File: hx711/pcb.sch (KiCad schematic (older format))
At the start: 31 parts, among them J1 RJ45_LED, J2 CONN_02X03_Odd_Even, J3 CONN_02X03_Odd_Even, J4 CONN_02X03_Odd_Even, J5 CONN_02X03_Odd_Even, U1 sp485, U2 RS485, U3 RS485, U4 20M, U5 MIC55, U6 USBLC6-4SC6, U7 USBLC6-4SC6

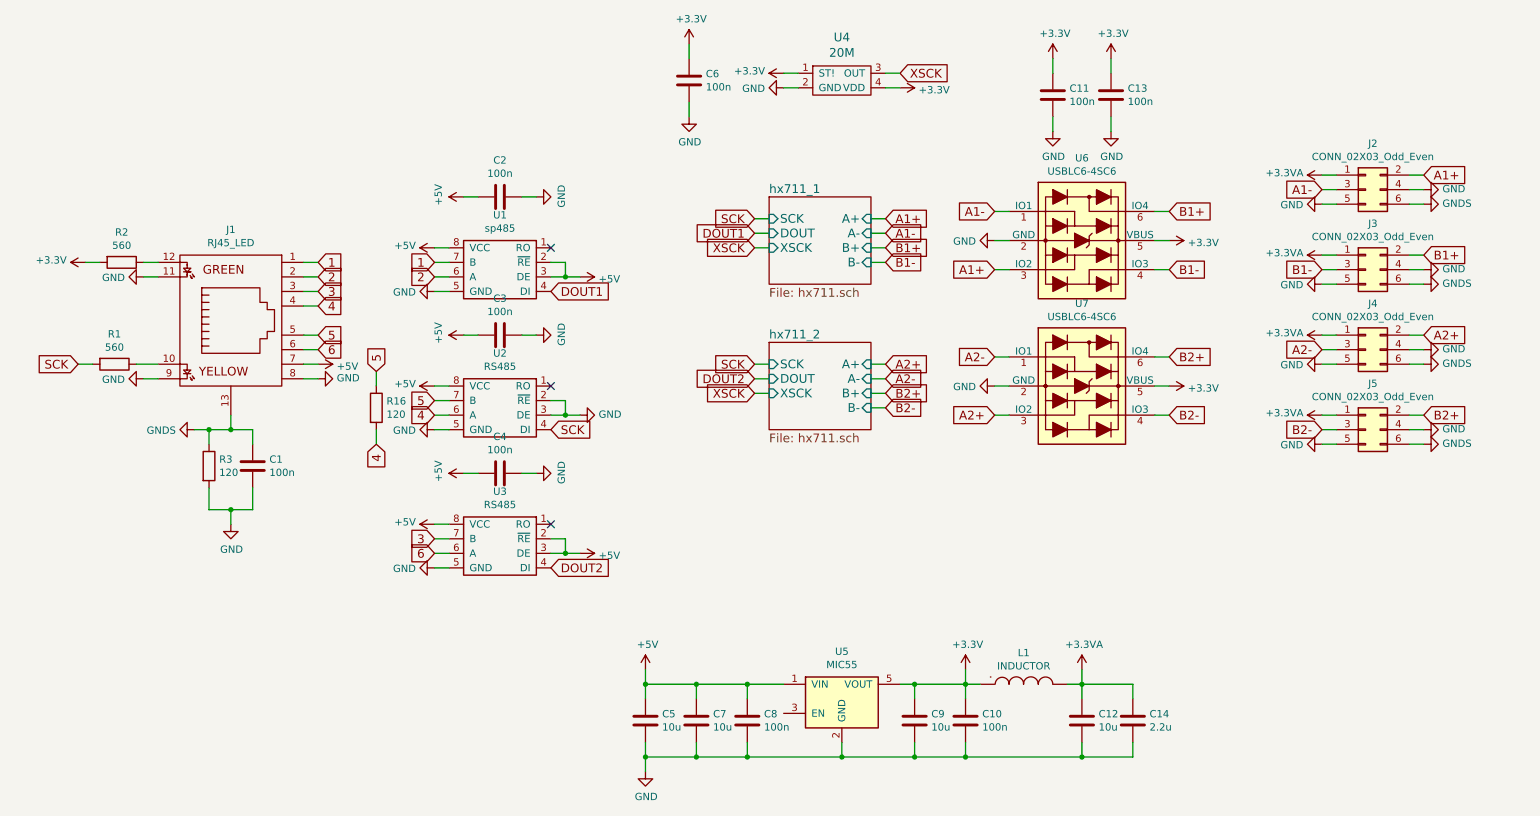
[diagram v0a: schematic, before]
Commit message: hx711
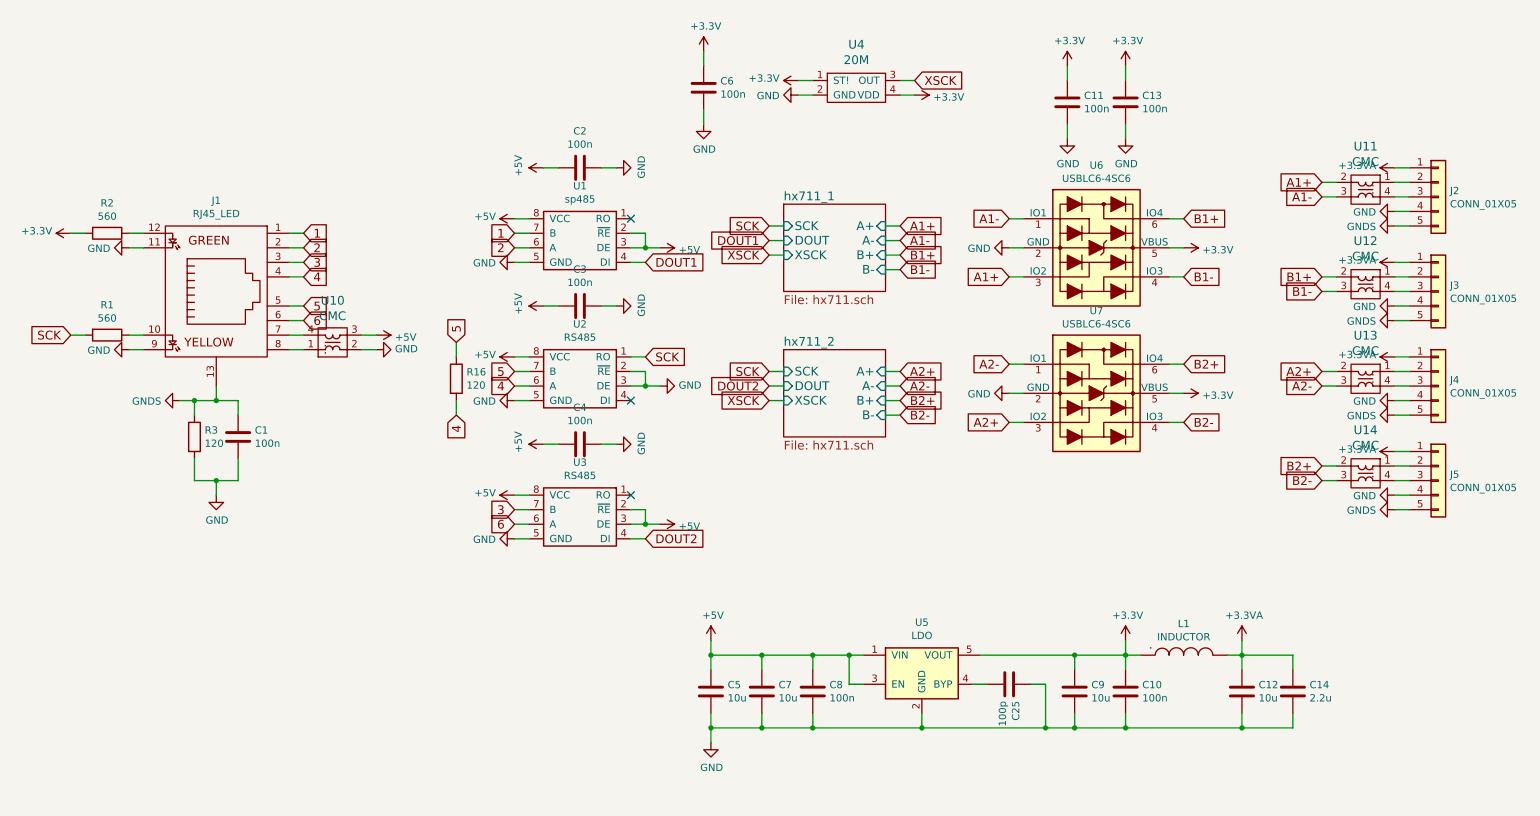
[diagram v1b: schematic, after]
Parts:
- removed J2, J3, J4, J5: CONN_02X03_Odd_Even, stmbl:Pin_Header_RM2.54_2x3_UP, symbol stmbl:CONN_02X03_Odd_Even
- removed U5: MIC55, stmbl:SOT-23-5, symbol stmbl:MIC55
- added C25: 100p, stmbl:C_0603, symbol stmbl:C
- added J2, J3, J4, J5: CONN_01X05, stmbl:Pin_Header_RM2.54_1x5_UP, symbol stmbl:CONN_01X05
- added U10, U11, U12, U13, U14: CMC, stmbl:CMC_0805, symbol stmbl:CMC
- added U5: LDO, stmbl:SOT-23-5, symbol stmbl:LDO
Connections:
- net +3.3VA: now also J2.1 (Pin_1), J3.1 (Pin_1), J4.1 (Pin_1), J5.1 (Pin_1)
- net +3V3: now also U5.5 (VOUT)
- net +5V: now also U10.3, U5.1 (VIN), U5.3 (EN); no longer J1.7
- net A1+: now also U11.2
- net A1-: now also U11.3
- net A2+: now also U13.2
- net A2-: now also U13.3
- net B1+: now also U12.2
- net B1-: now also U12.3
- net B2+: now also U14.2
- net B2-: now also U14.3
- net GND: now also C25.1, J2.4 (Pin_4), J3.4 (Pin_4), J4.4 (Pin_4), J5.4 (Pin_4), U10.2, U5.2 (GND); no longer J1.8
- net GNDS: now also J2.5 (Pin_5), J3.5 (Pin_5), J4.5 (Pin_5), J5.5 (Pin_5)
- net SCK: now also U2.1 (RO); no longer U2.4 (DI)
- new net: J2.2 (Pin_2), U11.1
- new net: J2.3 (Pin_3), U11.4
- new net: J1.7, U10.4
- new net: J1.8, U10.1
- new net: J3.2 (Pin_2), U12.1
- new net: J3.3 (Pin_3), U12.4
- new net: J4.2 (Pin_2), U13.1
- new net: J4.3 (Pin_3), U13.4
- new net: J5.2 (Pin_2), U14.1
- new net: J5.3 (Pin_3), U14.4
- new net: C25.2, U5.4 (BYP)
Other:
- moved on the sheet: C1, C10, C11, C12, C13, C14, C2, C3, C4, C5, C6, C7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
